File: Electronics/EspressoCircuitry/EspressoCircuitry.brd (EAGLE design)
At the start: 82.5 x 78.4 mm, 73 parts, among them IC1 TB6612FNG, IC2 TB6612FNG, IC3 TB6612FNG, J1 1X2-3.5MM, J10 1X2-3.5MM, J11 1X2-3.5MM, J12 1X2-3.5MM, J13 1X2-3.5MM, J14 1X2-3.5MM, J15 1X2-3.5MM, J16 1X2-3.5MM, J17 1X2-3.5MM, J18 1X2-3.5MM, J19 1X2-3.5MM, J2 1X2-3.5MM, J20 1X2-3.5MM, J21 1X2-3.5MM, J22 1X2-3.5MM, J23 1X2-3.5MM, J3 1X2-3.5MM, J4 1X2-3.5MM, J5 1X2-3.5MM, J6 1X2-3.5MM, J7 1X2-3.5MM, J8 1X2-3.5MM, J9 1X2-3.5MM, K1 G5LE, K2 G5LE, K3 G5LE, K4 G5LE

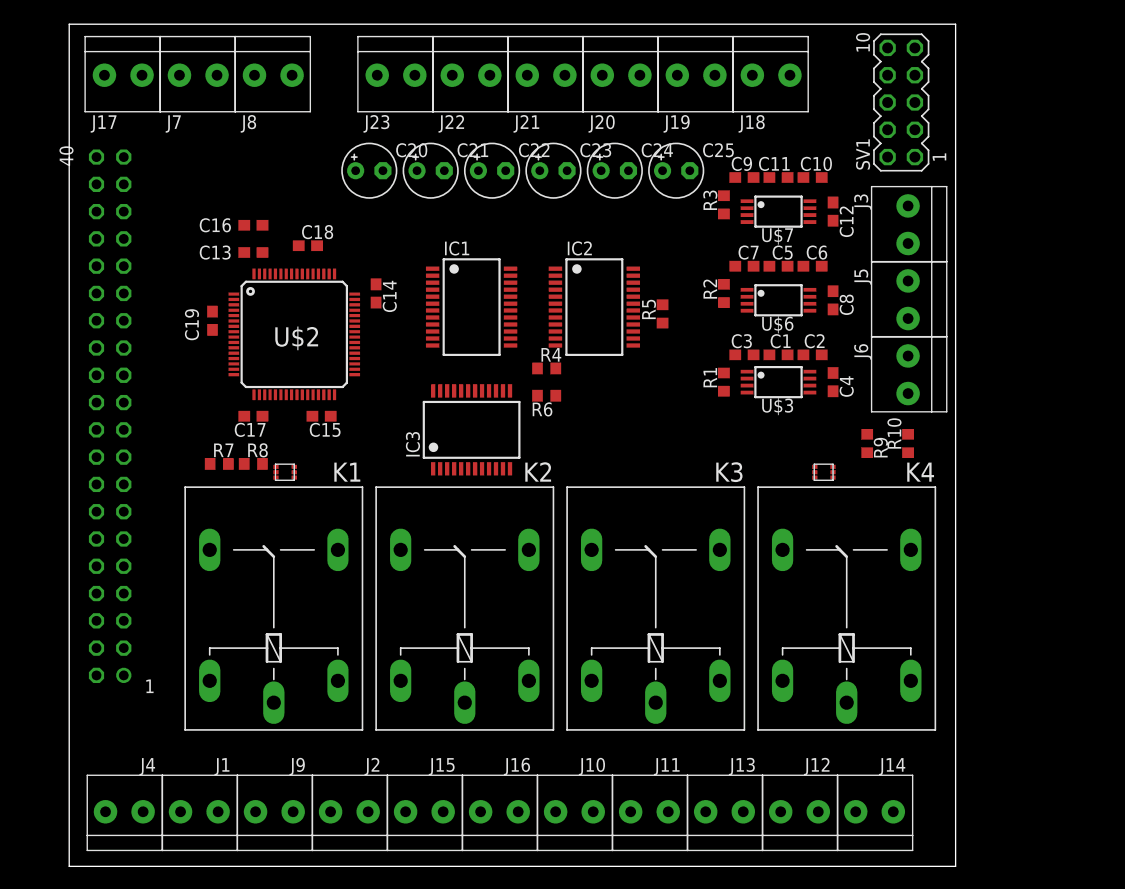
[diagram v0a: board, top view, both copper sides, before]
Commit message: Added updated PCB files
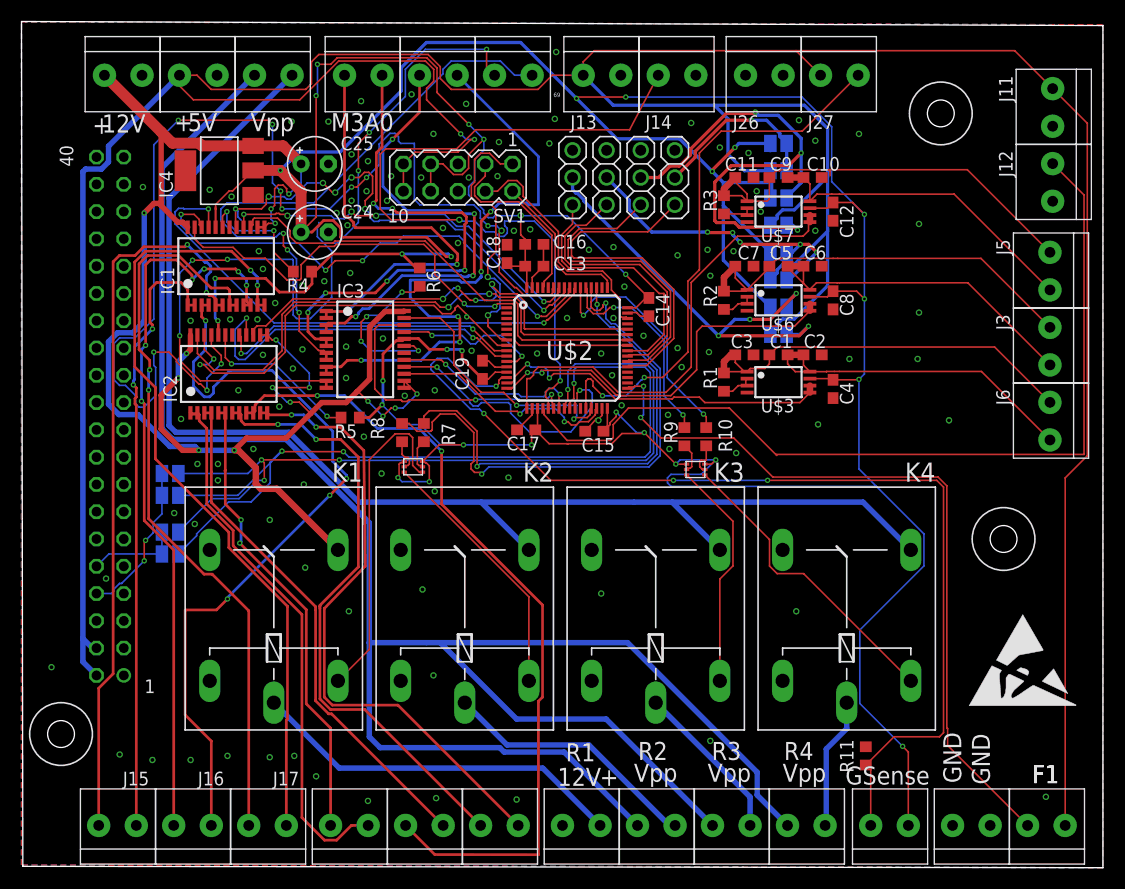
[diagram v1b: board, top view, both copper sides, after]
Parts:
- removed C20, C21, C22, C23: 10u, rcl:E2,5-5
- added IC4: REG1117, burr-brown:SOT223
- added J24, J25, J26, J27, J28: 1X2-3.5MM, adafruit:1X2-3.5MM
- added JP1, JP2, JP3, JP4: (no value), adafruit:1X03
- added R11: 10k, rcl:R0603
- added SJ1, SJ10, SJ11, SJ12, SJ2, SJ3, SJ4, SJ5, SJ6, SJ7, SJ8, SJ9: (no value), jumper:SJ
- added U$10, U$11, U$9: (no value), special:DRIL-2,5
- added U$8: (no value), logo:ESD_10.00
- C24, C25: value 10u -> 100u
- moved J7 81.8 mm to (54.6, 3.81), turned to 0 degrees
- moved J18 80.2 mm to (26.0, 3.81), turned to 0 degrees
- moved J11 75.5 mm to (91.6, 70.6), turned to 90 degrees
- moved J19 74.3 mm to (33.0, 3.81), turned to 0 degrees
- moved J17 71.1 mm to (18.4, 3.81), turned to 0 degrees
- moved J14 71.0 mm to (56.6, 73.7), turned to 180 degrees
- moved J20 70.8 mm to (40.0, 3.81), turned to 0 degrees
- moved J2 70.0 mm to (12.1, 73.7), turned to 180 degrees
- moved J13 69.5 mm to (49.7, 73.7), turned to 180 degrees
- moved J1 68.9 mm to (5.08, 73.7), turned to 180 degrees
- moved J12 63.1 mm to (91.6, 63.6), turned to 90 degrees
- moved J4 42.6 mm to (47.6, 3.81)
- moved J9 42.6 mm to (61.6, 3.81)
- moved SV1 41.9 mm to (36.2, 64.1), turned to 180 degrees
- moved IC2 34.6 mm to (14.9, 45.8), turned to 0 degrees
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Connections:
- removed net SWCLK: SV1.2
- new net FLOW1: J25.2, U$2.33
- new net FLOW2: J27.2, U$2.28
- new net GROUND_SENSE: J24.2, R11.2, U$2.14
- new net N$44: JP1.2, SJ1.2, SJ2.2
- new net N$45: JP2.2, SJ3.2, SJ4.2
- new net N$46: JP3.2, SJ5.2, SJ6.2
- new net N$47: JP4.2, SJ7.2, SJ8.2
- new net N$48: SJ11.1, SJ12.1, U$1.10
- new net SERVO1: JP1.1, U$2.37
- new net SERVO2: JP2.1, U$2.38
- new net SERVO3: JP3.1, U$2.39
- new net SERVO4: JP4.1, U$2.40
- net +12V: now also IC4.3; no longer C21.+, C23.+
- net +3V3: now also C13.1, IC4.2, J24.1, SJ1.1, SJ3.1, SJ5.1, SJ7.1; no longer C20.+, C22.+
- net +5V: now also J25.1, J27.1, SJ2.1, SJ4.1, SJ6.1, SJ8.1
- net GND: now also C18.2, IC4.1, J26.1, J26.2, J28.1, J28.2, JP1.3, JP2.3, JP3.3, JP4.3, R11.1; no longer C20.-, C21.-, C22.-, C23.-
- net M1_AIN1: now also U$2.55
- net M1_AIN2: now also U$2.56
- net M1_BIN1: now also U$2.57
- net M1_BIN2: now also U$2.58
- net M1_PWMA: now also U$2.41
- net M1_PWMB: now also U$2.42
- net M2_AIN1: now also U$2.59
- net M2_AIN2: now also U$2.8
- net M2_BIN1: now also U$2.9
- net M2_BIN2: now also U$2.10
- net M2_PWMA: now also U$2.43
- net M2_PWMB: now also U$2.44
- net M3_AIN1: now also U$2.11
- net M3_AIN2: now also U$2.22
- net M3_BIN1: now also U$2.23
- net M3_BIN2: now also U$2.26
- net M3_PWMA: now also U$2.29
- net M3_PWMB: now also U$2.30
- net N$1: now also SJ10.1, SJ9.1, U$1.8; no longer U$2.20
- net PRESSURE1: now also U$2.20
- net PRESSURE2: now also U$2.21
- net RX: now also SJ11.2, SJ9.2; no longer U$1.8
- net SWDCLK: now also SV1.2
- net TEMP1: now also U$2.15
- net TEMP2: now also U$2.16
- net TEMP3: now also U$2.17
- net TX: now also SJ10.2, SJ12.2; no longer U$1.10
- net ~RELAY1: now also U$2.51
- net ~RELAY2: now also U$2.52
- net ~RELAY3: now also U$2.53
- net ~RELAY4: now also U$2.54
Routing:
- net +3V3: track 0.00 -> 456.7 mm, vias 0 -> 31
- net +5V: track 0.00 -> 344.2 mm, vias 0 -> 2
- net V-: track 0.00 -> 187.4 mm
- net +12V: track 0.00 -> 155.7 mm, vias 0 -> 16
- net V+: track 0.00 -> 123.8 mm
- net M2_AIN1: track 0.00 -> 109.6 mm, vias 0 -> 11
- net GROUND_SENSE: track 0.00 -> 98.8 mm, vias 0 -> 4
- net PRESSURE1: track 0.00 -> 84.2 mm
- net N$37: track 0.00 -> 82.7 mm, vias 0 -> 6
- net TX: track 0.00 -> 79.4 mm, vias 0 -> 3
- net RX: track 0.00 -> 76.9 mm, vias 0 -> 4
- net N$28: track 0.00 -> 76.4 mm, vias 0 -> 2
- net N$21: track 0.00 -> 74.5 mm, vias 0 -> 2
- net N$15: track 0.00 -> 72.2 mm, vias 0 -> 4
- net PRESSURE2: track 0.00 -> 71.3 mm, vias 0 -> 2
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- added copper zone on layer 1, net GND
- added copper zone on layer 16, net GND
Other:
- board size 82.5 x 78.4 mm -> 100.7 x 78.8 mm
- board text added: "+"
- board text added: "12V"
- board text added: "5V"
- board text added: "69"
- board text added: "Aaron Pabst"
- board text added: "F1"
- board text added: "GND"
- board text added: "GSense"
- board text added: "M3A0"
- board text added: "R1"
- board text added: "R2"
- board text added: "R3"
- board text added: "R4"
- board text added: "Vpp"
